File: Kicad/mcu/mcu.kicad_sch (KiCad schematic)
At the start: 9 parts, among them IC301 PIC16F1778, K301 MCU 1, K302 ICSP, K303 MCU 2

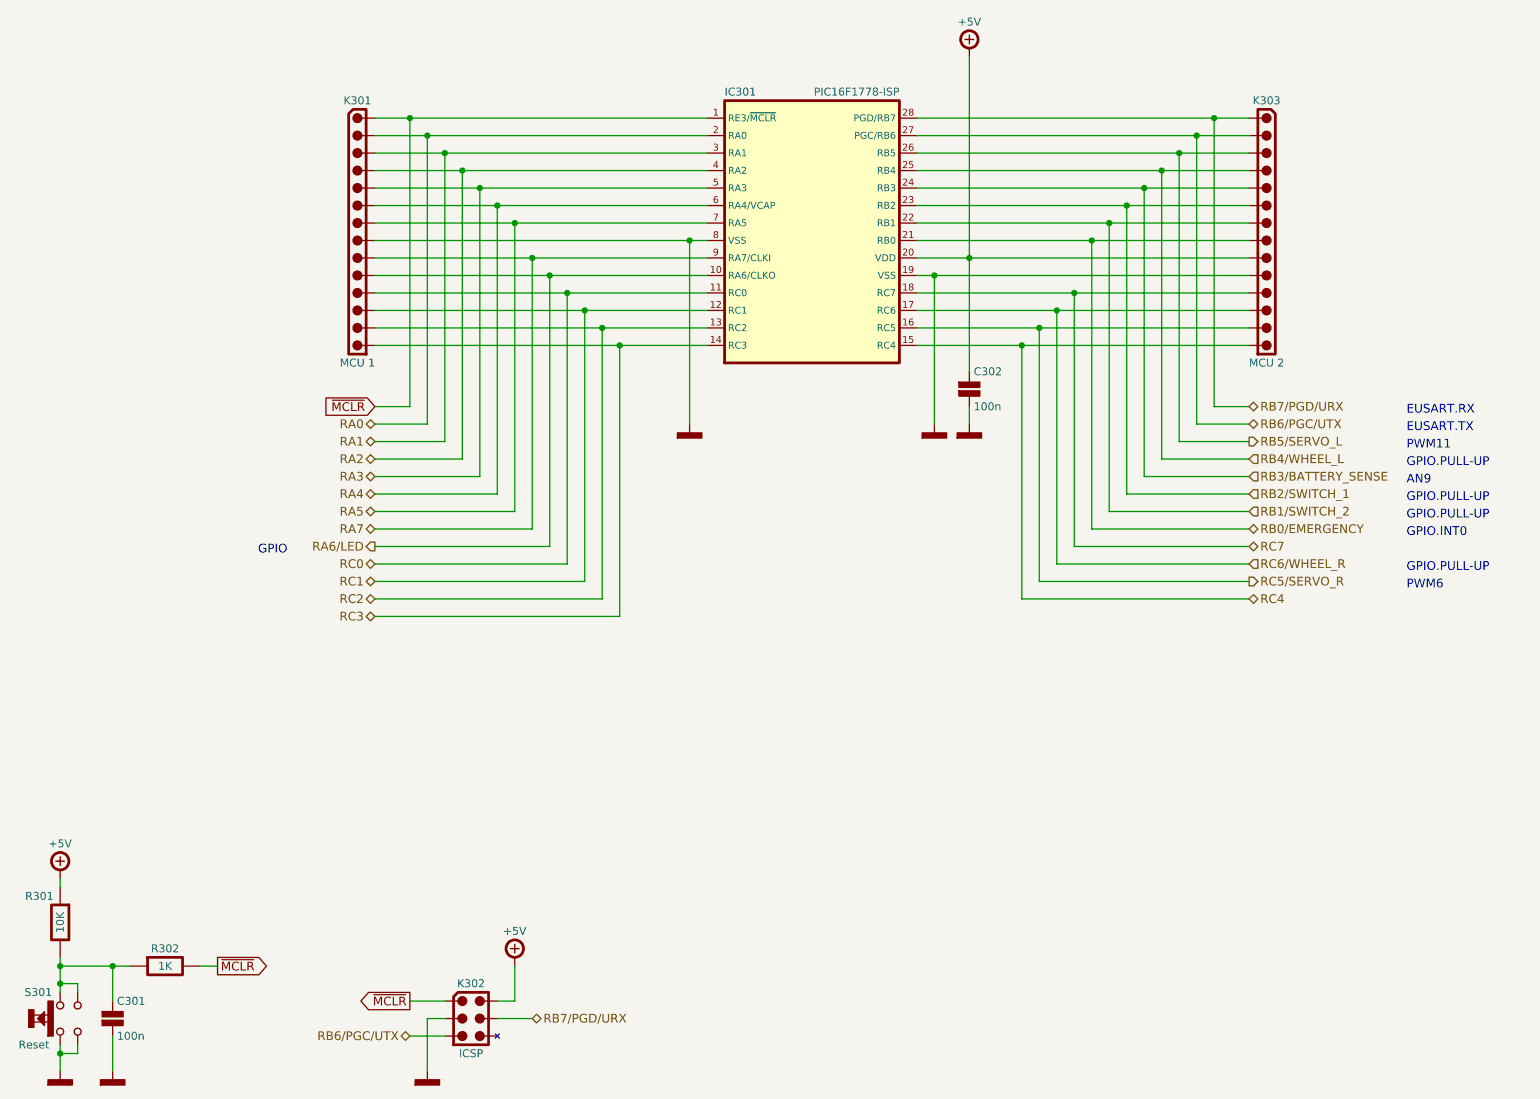
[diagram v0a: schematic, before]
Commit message: Update MCU
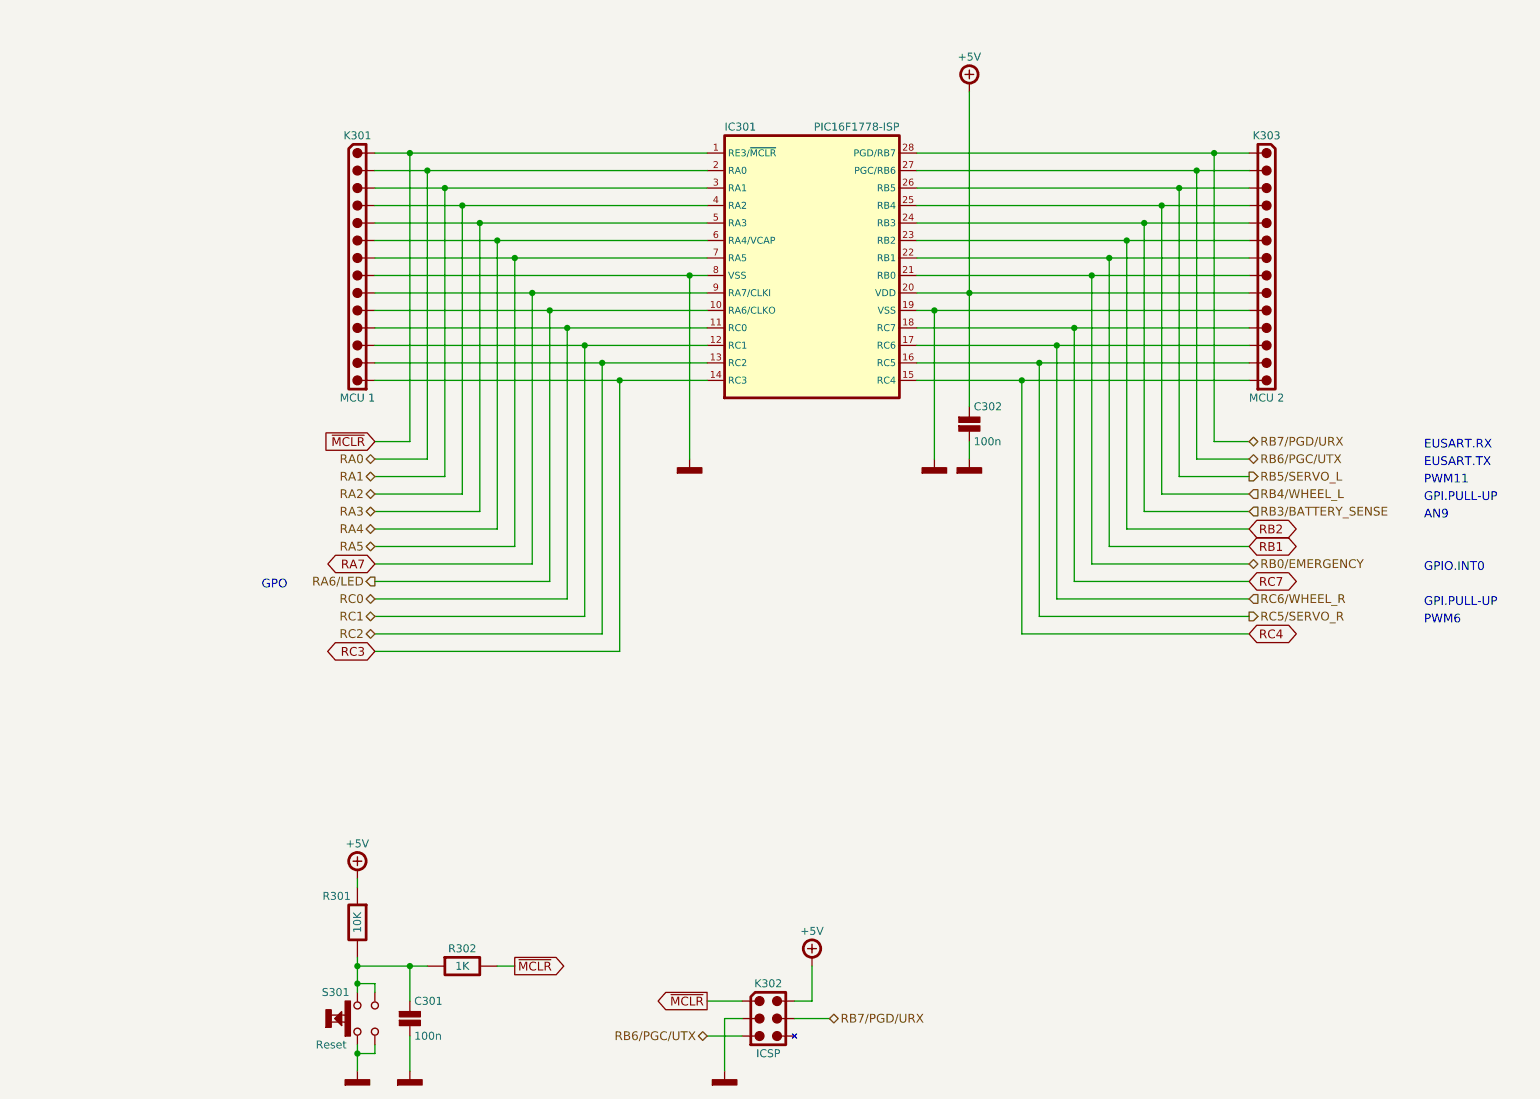
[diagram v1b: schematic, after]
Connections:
- net RB1/SWITCH_2 renamed RB1
- net RB2/SWITCH_1 renamed RB2
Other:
- note added: "GPI.PULL-UP"
- note added: "GPO"
- note removed: "GPIO"
- note removed: "GPIO.PULL-UP"
- moved on the sheet: C301, C302, IC301, K301, K302, K303, R301, R302, S301
